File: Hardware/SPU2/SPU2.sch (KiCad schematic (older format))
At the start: 736 parts, among them J1 Conn_Coaxial, J2 Conn_02x13_Counter_Clockwise, J3 Conn_01x02, J4 Conn_01x04_Male, Q2 BC547, Q3 BC547, Q4 BC547, SW1 SW_Push, SW2 SW_SPDT, SW3 SW_DIP_x02, U1 74LS86, U10 74LS08, U11 74LS173, U12 74LS173, U13 74LS161, U14 74LS161, U15 74LS161, U16 74LS173, U17 74LS173, U18 NE555, U19 74LS173, U2 74LS86, U20 74LS173, U21 74LS173, U22 74LS173, U23 74LS173, U24 74LS173, U25 74LS245, U26 M84Z02, U27 M84Z02, U28 74LS245, U29 74LS00, U3 74LS245, U30 28c64, U31 28c64, U32 74LS245, U33 74LS245, U34 74LS245, U35 74LS245, U36 74LS245, U37 74LS08, U38 74HCT574, U39 74HCT574, U4 74LS283, U40 74LS161, U41 74LS04, U42 74LS08, U43 NE555, U44 NE555, U45 74HCT574, U46 74HCT574, U47 74HCT574, U48 74HCT574, U49 74HCT574, U5 74LS283, U50 74HCT574, U51 74HCT574, U52 74HCT574, U53 74HCT574, U54 74HCT574, U55 74HCT574, U56 74HCT574, U57 74HCT574, U58 74HCT574, U59 74HCT574, U6 4077, U60 74HCT574, U61 INTEL2716, U62 74LS08, U63 INTEL2716, U64 74LS08, U65 74LS08, U66 74LS08, U67 74LS08, U68 INTEL2716, U69 CD4514B, U7 4077, U70 74LS157, U76 74LS157, U77 74LS157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

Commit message: done stuff
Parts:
- gave numbers to parts that had none: 10
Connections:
- net GND: no longer D122.1 (K), D123.1 (K), D124.1 (K), D125.1 (K), D126.1 (K), D127.1 (K), D128.1 (K), D129.1 (K)
- net RAMOBUS0: now also U70.2 (I0a); no longer U70.3 (I1a)
- net RAMOBUS1: now also U70.5 (I0b); no longer U70.6 (I1b)
- net RAMOBUS10: now also U77.11 (I0c); no longer U77.10 (I1c)
- net RAMOBUS11: now also U77.14 (I0d); no longer U77.13 (I1d)
- net RAMOBUS12: now also U78.2 (I0a); no longer U78.3 (I1a)
- net RAMOBUS13: now also U78.5 (I0b); no longer U78.6 (I1b)
- net RAMOBUS14: now also U78.11 (I0c); no longer U78.10 (I1c)
- net RAMOBUS15: now also U78.14 (I0d); no longer U78.13 (I1d)
- net RAMOBUS2: now also U70.11 (I0c); no longer U70.10 (I1c)
- net RAMOBUS3: now also U70.14 (I0d); no longer U70.13 (I1d)
- net RAMOBUS4: now also U76.2 (I0a); no longer U76.3 (I1a)
- net RAMOBUS5: now also U76.5 (I0b); no longer U76.6 (I1b)
- net RAMOBUS6: now also U76.11 (I0c); no longer U76.10 (I1c)
- net RAMOBUS7: now also U76.14 (I0d); no longer U76.13 (I1d)
- net RAMOBUS8: now also U77.2 (I0a); no longer U77.3 (I1a)
- net RAMOBUS9: now also U77.5 (I0b); no longer U77.6 (I1b)
- net ROM0: now also U70.3 (I1a); no longer U70.2 (I0a)
- net ROM1: now also U70.6 (I1b); no longer U70.5 (I0b)
- net ROM10: now also U77.10 (I1c); no longer U77.11 (I0c)
- net ROM11: now also U77.13 (I1d); no longer U77.14 (I0d)
- net ROM12: now also U78.3 (I1a); no longer U78.2 (I0a)
- net ROM13: now also U78.6 (I1b); no longer U78.5 (I0b)
- net ROM14: now also U78.10 (I1c); no longer U78.11 (I0c)
- net ROM15: now also U78.13 (I1d); no longer U78.14 (I0d)
- net ROM2: now also U70.10 (I1c); no longer U70.11 (I0c)
- net ROM3: now also U70.13 (I1d); no longer U70.14 (I0d)
- net ROM4: now also U76.3 (I1a); no longer U76.2 (I0a)
- net ROM5: now also U76.6 (I1b); no longer U76.5 (I0b)
- net ROM6: now also U76.10 (I1c); no longer U76.11 (I0c)
- net ROM7: now also U76.13 (I1d); no longer U76.14 (I0d)
- net ROM8: now also U77.3 (I1a); no longer U77.2 (I0a)
- net ROM9: now also U77.6 (I1b); no longer U77.5 (I0b)
- net NE555_CLK: now reaches R125.2, U41.8
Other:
- note added: "RAM (LEDs)\n"
- note added: "excess NAND gates (RAM)\n"
- note removed: "architecture diagram\n\n"
- note removed: "ram leds"
- note removed: "übrige nand gates (für ram)"
- moved on the sheet: C1, C10, C11, C12, C13, C14, C15, C16, C17, C18, C19, C22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

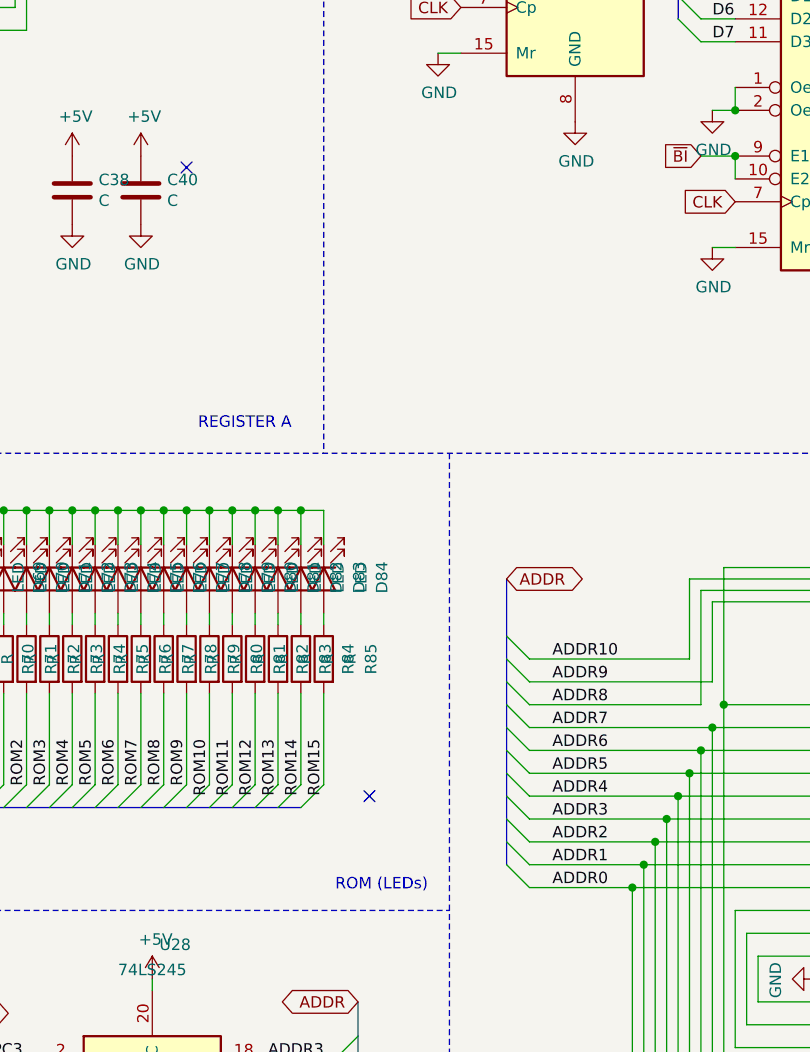
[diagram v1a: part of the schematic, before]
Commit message: existance is pain
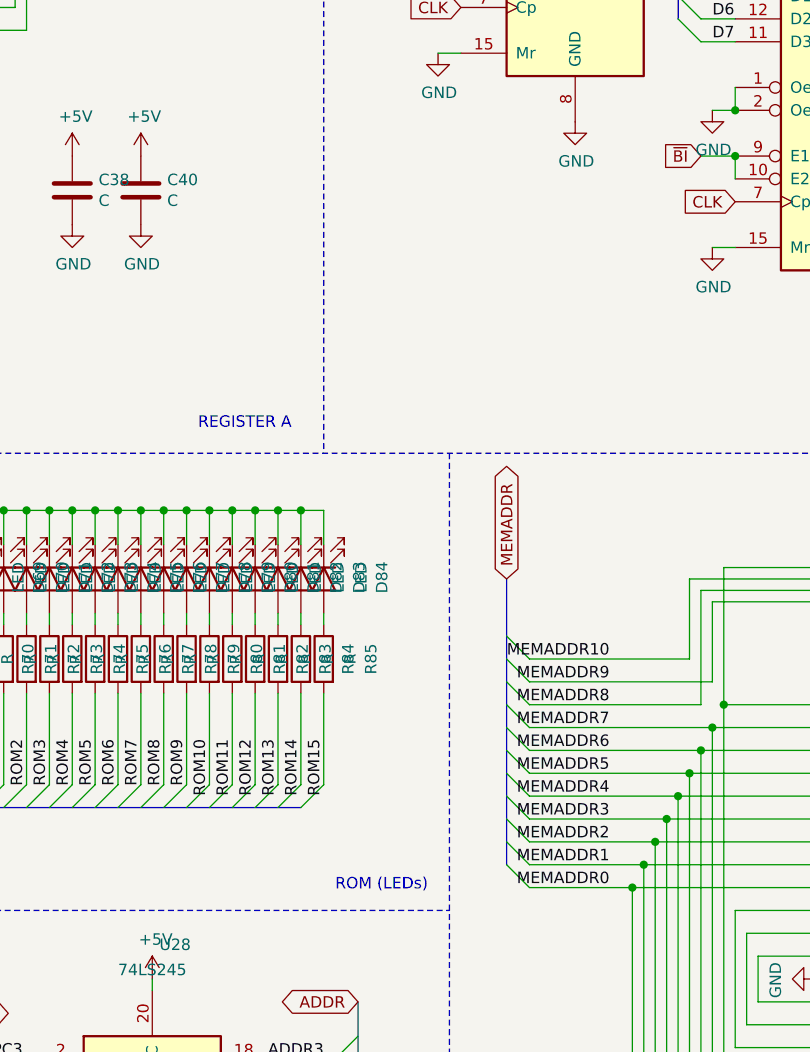
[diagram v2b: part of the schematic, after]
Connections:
- net ADDR0: no longer U30.10 (A0), U31.10 (A0)
- net ADDR1: no longer U30.9 (A1), U31.9 (A1)
- net ADDR10: no longer U30.21 (A10), U31.21 (A10)
- net ADDR2: no longer U30.8 (A2), U31.8 (A2)
- net ADDR3: no longer U30.7 (A3), U31.7 (A3)
- net ADDR4: no longer U30.6 (A4), U31.6 (A4)
- net ADDR5: no longer U30.5 (A5), U31.5 (A5)
- net ADDR6: no longer U30.4 (A6), U31.4 (A6)
- net ADDR7: no longer U30.3 (A7), U31.3 (A7)
- net ADDR8: no longer U30.25 (A8), U31.25 (A8)
- net ADDR9: no longer U30.24 (A9), U31.24 (A9)
- net MEMADDR0: now also U30.10 (A0), U31.10 (A0)
- net MEMADDR1: now also U30.9 (A1), U31.9 (A1)
- net MEMADDR10: now also U30.21 (A10), U31.21 (A10)
- net MEMADDR2: now also U30.8 (A2), U31.8 (A2)
- net MEMADDR3: now also U30.7 (A3), U31.7 (A3)
- net MEMADDR4: now also U30.6 (A4), U31.6 (A4)
- net MEMADDR5: now also U30.5 (A5), U31.5 (A5)
- net MEMADDR6: now also U30.4 (A6), U31.4 (A6)
- net MEMADDR7: now also U30.3 (A7), U31.3 (A7)
- net MEMADDR8: now also U30.25 (A8), U31.25 (A8)
- net MEMADDR9: now also U30.24 (A9), U31.24 (A9)
- no-connect marks 41 -> 39
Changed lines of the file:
@@
 	1    0    0    -1
 $EndComp
-NoConn ~ 15450 5950
-NoConn ~ 14650 3200
 $Comp
 L Device:C C84
@@
 Wire Wire Line
 	16650 8200 16650 6250
-Connection ~ 16650 6250
 Wire Wire Line
 	16600 8300 16600 6350
 Connection ~ 16600 6350
-Text GLabel 16050 5000 2    50   BiDi ~ 0
-ADDR
-Text Label 16250 5350 0    50   ~ 0
-ADDR10
-Text Label 16250 5450 0    50   ~ 0
-ADDR9
-Text Label 16250 5550 0    50   ~ 0
-ADDR8
-Entry Wire Line
-	16150 5350 16050 5250
-Entry Wire Line
-	16150 5450 16050 5350
-Entry Wire Line
-	16150 5550 16050 5450
-Text Label 16250 5650 0    50   ~ 0
-ADDR7
-Text Label 16250 5750 0    50   ~ 0
-ADDR6
-Text Label 16250 5850 0    50   ~ 0
-ADDR5
-Text Label 16250 5950 0    50   ~ 0
-ADDR4
-Entry Wire Line
-	16150 5650 16050 5550
-Entry Wire Line
-	16150 5750 16050 5650
-Entry Wire Line
-	16150 5850 16050 5750
-Entry Wire Line
-	16150 5950 16050 5850
-Entry Wire Line
-	16150 6350 16050 6250
-Entry Wire Line
-	16150 6250 16050 6150
-Entry Wire Line
-	16150 6150 16050 6050
-Entry Wire Line
-	16150 6050 16050 5950
-Text Label 16250 6350 0    50   ~ 0
-ADDR0
-Text Label 16250 6250 0    50   ~ 0
-ADDR1
-Text Label 16250 6150 0    50   ~ 0
-ADDR2
-Text Label 16250 6050 0    50   ~ 0
-ADDR3
 Wire Wire Line
 	16150 6350 16600 6350
 Wire Wire Line
-	16150 6250 16650 6250
-Wire Wire Line
 	16150 6150 16700 6150
 Wire Wire Line
@@
 EndData
 $EndBitmap
+Entry Wire Line
+	16150 5350 16050 5250
+Entry Wire Line
+	16150 5450 16050 5350
+Entry Wire Line
+	16150 5550 16050 5450
+Entry Wire Line
+	16150 5650 16050 5550
+Entry Wire Line
+	16150 5750 16050 5650
+Entry Wire Line
+	16150 5850 16050 5750
+Entry Wire Line
+	16150 5950 16050 5850
+Entry Wire Line
+	16150 6350 16050 6250
+Entry Wire Line
+	16150 6250 16050 6150
+Entry Wire Line
+	16150 6150 16050 6050
+Entry Wire Line
+	16150 6050 16050 5950
+Text GLabel 16050 5000 1    50   BiDi ~ 0
+MEMADDR
+Text Label 16500 6350 2    50   ~ 0
+MEMADDR0
+Text Label 16500 6250 2    50   ~ 0
+MEMADDR1
+Text Label 16500 6150 2    50   ~ 0
+MEMADDR2
+Text Label 16500 6050 2    50   ~ 0
+MEMADDR3
+Text Label 16500 5950 2    50   ~ 0
+MEMADDR4
+Text Label 16500 5850 2    50   ~ 0
+MEMADDR5
+Text Label 16500 5750 2    50   ~ 0
+MEMADDR6
+Text Label 16500 5650 2    50   ~ 0
+MEMADDR7
+Text Label 16500 5550 2    50   ~ 0
+MEMADDR8
+Text Label 16500 5450 2    50   ~ 0
+MEMADDR9
+Text Label 16500 5350 2    50   ~ 0
+MEMADDR10
+Wire Wire Line
+	16150 6250 16650 6250
 Wire Bus Line
 	29950 14350 29950 14550
@@
 	4050 4750 4050 5650
 Wire Bus Line
-	16050 5000 16050 6250
-Wire Bus Line
 	12300 10350 12300 11800
 Wire Bus Line
@@
 	21950 6250 21950 7250
 Wire Bus Line
+	16050 5000 16050 6250
+Wire Bus Line
 	22500 13550 22500 21900
 Wire Bus Line
@@
 Wire Bus Line
 	13500 6000 15150 6000
+Connection ~ 16650 6250
 $EndSCHEMATC
